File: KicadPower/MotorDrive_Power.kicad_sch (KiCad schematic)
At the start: 9 parts, among them P4 Connector, P5 Connector, P7 Connector, P8 Connector, P9 Connector

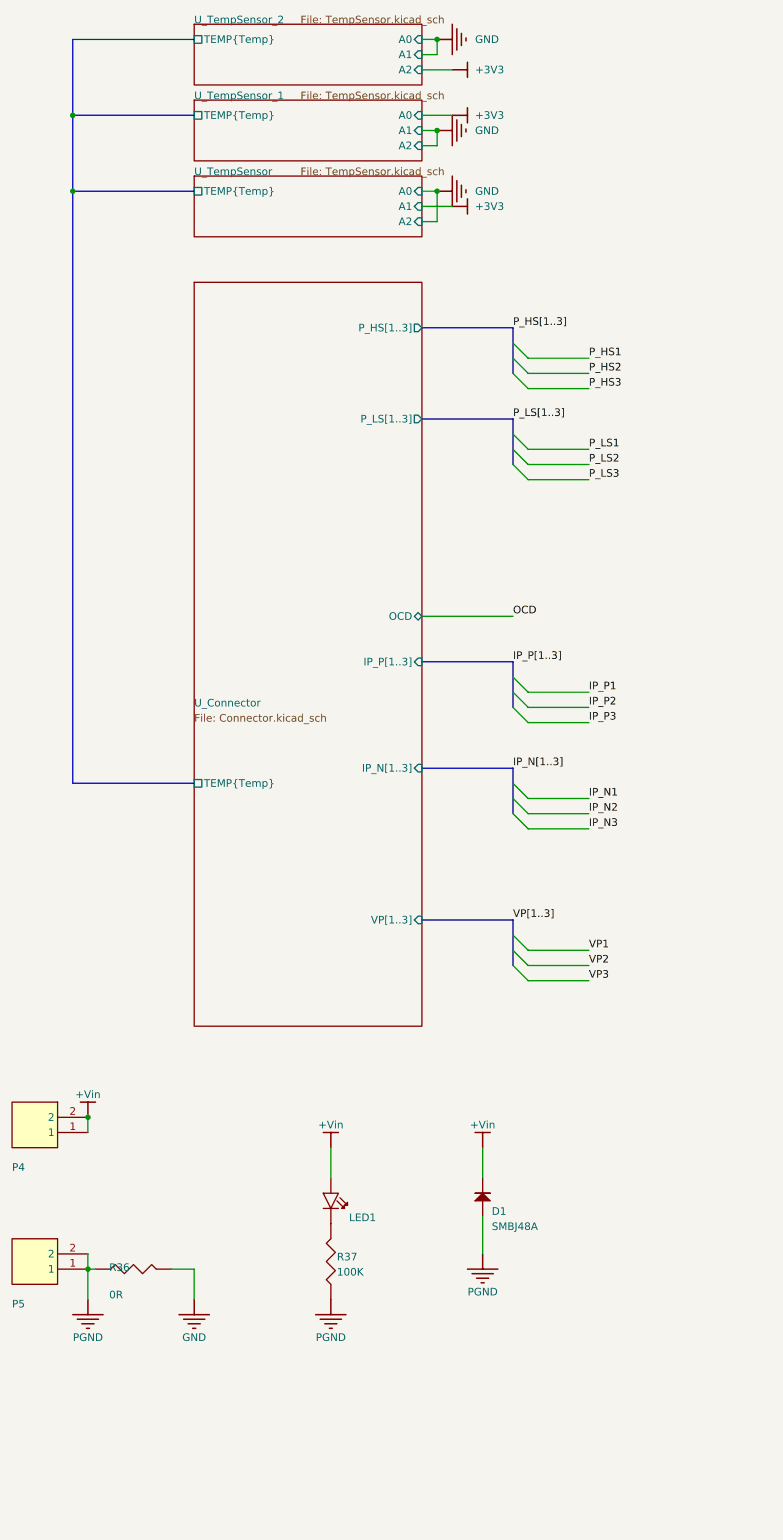
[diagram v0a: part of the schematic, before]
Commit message: minor changes
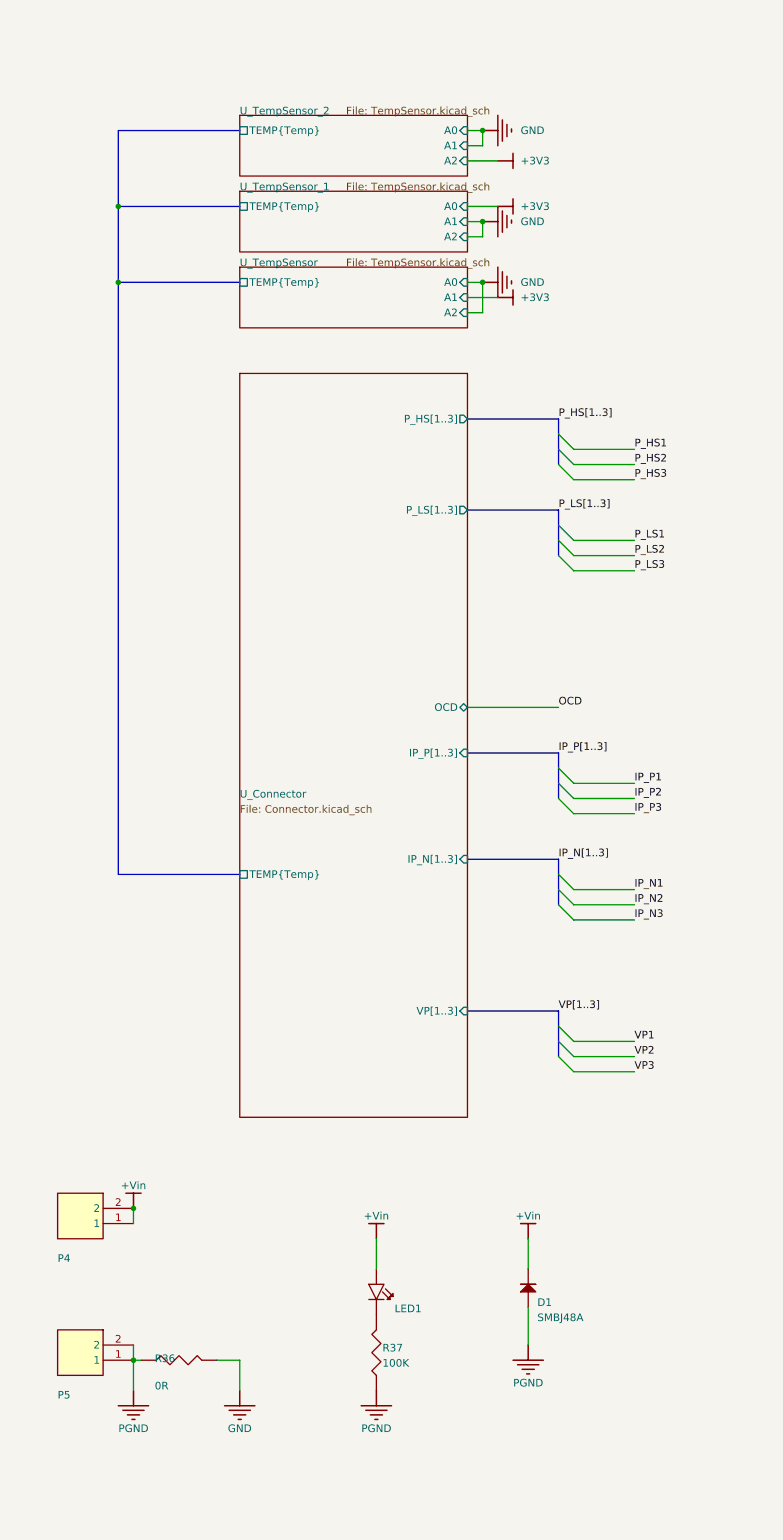
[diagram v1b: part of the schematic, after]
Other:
- moved on the sheet: D1, LED1, P4, P5, R36, R37
